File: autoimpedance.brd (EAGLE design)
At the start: 32.1 x 50.8 mm, 42 parts, among them IC1 AD5933, IC2 LM234, IC3 AD5245, Q1 DMG2307L-7

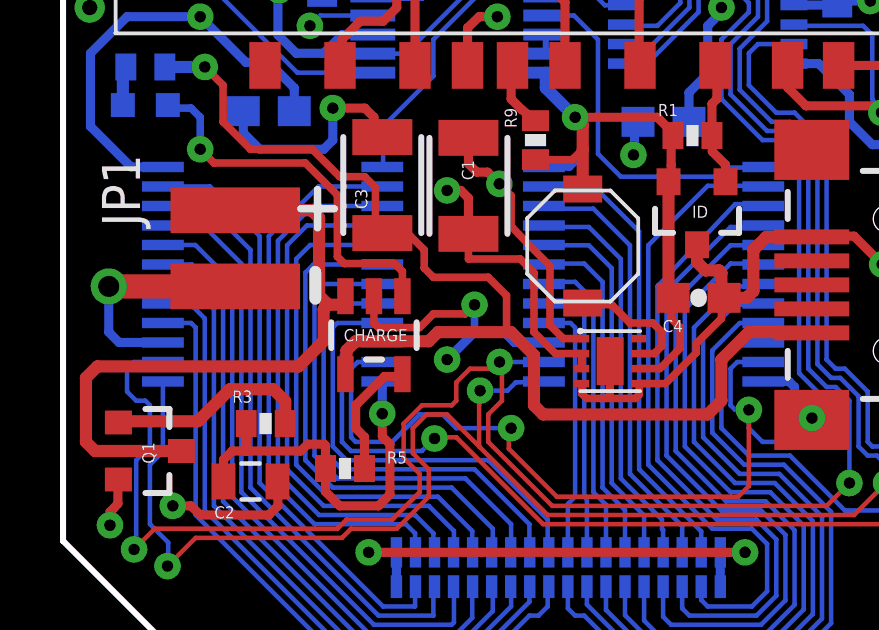
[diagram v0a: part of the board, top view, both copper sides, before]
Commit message: Add Gerber files and .cam
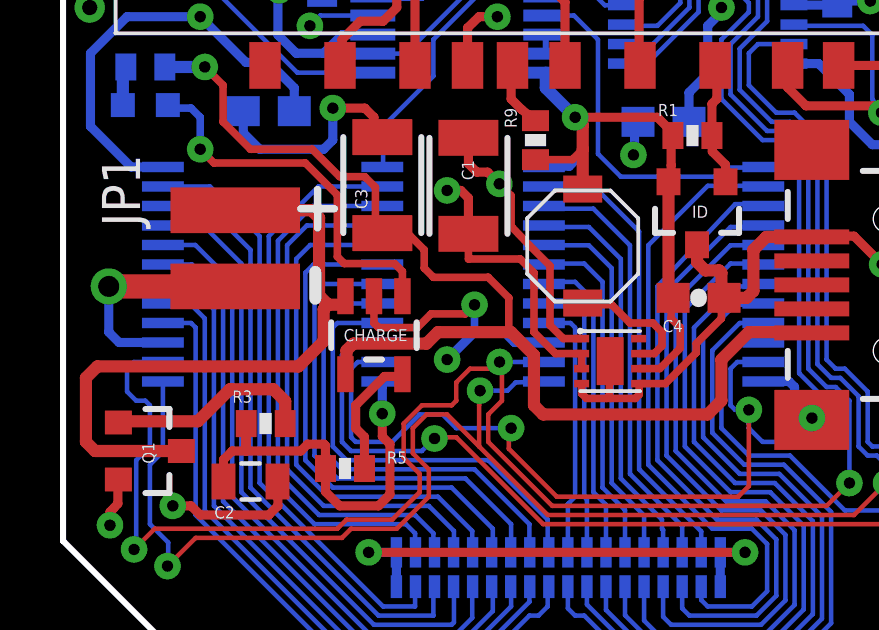
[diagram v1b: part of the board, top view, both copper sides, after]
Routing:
- net VIN: track 27.9 -> 29.5 mm
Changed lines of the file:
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@@
 <layer number="1" name="Top" color="4" fill="1" visible="no" active="yes"/>
 <layer number="2" name="Route2" color="11" fill="1" visible="no" active="yes"/>
-<layer number="3" name="Route3" color="8" fill="1" visible="no" active="yes"/>
+<layer number="3" name="Route3" color="8" fill="1" visible="yes" active="yes"/>
 <layer number="4" name="Route4" color="1" fill="4" visible="no" active="no"/>
 <layer number="5" name="Route5" color="4" fill="4" visible="no" active="no"/>
@@
 <layer number="15" name="Route15" color="4" fill="6" visible="no" active="no"/>
 <layer number="16" name="Bottom" color="1" fill="1" visible="no" active="yes"/>
-<layer number="17" name="Pads" color="2" fill="1" visible="no" active="yes"/>
-<layer number="18" name="Vias" color="2" fill="1" visible="no" active="yes"/>
+<layer number="17" name="Pads" color="2" fill="1" visible="yes" active="yes"/>
+<layer number="18" name="Vias" color="2" fill="1" visible="yes" active="yes"/>
 <layer number="19" name="Unrouted" color="15" fill="1" visible="no" active="yes"/>
 <layer number="20" name="Dimension" color="15" fill="1" visible="no" active="yes"/>
-<layer number="21" name="tPlace" color="3" fill="1" visible="no" active="yes"/>
+<layer number="21" name="tPlace" color="3" fill="1" visible="yes" active="yes"/>
 <layer number="22" name="bPlace" color="5" fill="1" visible="yes" active="yes"/>
 <layer number="23" name="tOrigins" color="15" fill="1" visible="no" active="yes"/>
 <layer number="24" name="bOrigins" color="15" fill="1" visible="no" active="yes"/>
-<layer number="25" name="tNames" color="3" fill="1" visible="no" active="yes"/>
+<layer number="25" name="tNames" color="3" fill="1" visible="yes" active="yes"/>
 <layer number="26" name="bNames" color="5" fill="1" visible="yes" active="yes"/>
-<layer number="27" name="tValues" color="3" fill="1" visible="no" active="yes"/>
+<layer number="27" name="tValues" color="3" fill="1" visible="yes" active="yes"/>
 <layer number="28" name="bValues" color="5" fill="1" visible="yes" active="yes"/>
 <layer number="29" name="tStop" color="7" fill="1" visible="no" active="yes"/>
@@
 <wire x1="10.3632" y1="13.2381" x2="10.3632" y2="12.3444" width="0.254" layer="1"/>
 <wire x1="10.3632" y1="12.3444" x2="10.5156" y2="12.192" width="0.254" layer="1"/>
-<wire x1="10.5156" y1="12.192" x2="11.8872" y2="12.192" width="0.254" layer="1"/>
-<wire x1="11.8872" y1="12.192" x2="12.3444" y2="12.6492" width="0.254" layer="1"/>
-<wire x1="12.3444" y1="12.6492" x2="13.4112" y2="12.6492" width="0.254" layer="1"/>
+<wire x1="10.5156" y1="12.192" x2="11.811" y2="12.192" width="0.254" layer="1"/>
+<wire x1="11.811" y1="12.192" x2="12.2682" y2="12.6492" width="0.254" layer="1"/>
+<wire x1="12.2682" y1="12.6492" x2="13.4112" y2="12.6492" width="0.254" layer="1"/>
 <wire x1="13.4112" y1="12.6492" x2="13.716" y2="12.954" width="0.254" layer="1"/>
 <wire x1="5.7404" y1="13.5636" x2="1.524" y2="13.5636" width="0.8128" layer="1"/>
@@
 <wire x1="15.24" y1="14.478" x2="13.513" y2="14.478" width="0.254" layer="1"/>
 <wire x1="13.513" y1="14.478" x2="13.5128" y2="15.3164" width="0.254" layer="1"/>
-<wire x1="1.5646" y1="5.6032" x2="7.1272" y2="8.956" width="0.6096" layer="3"/>
-<wire x1="7.1272" y1="8.956" x2="12.8016" y2="14.6304" width="0.6096" layer="3"/>
-<wire x1="12.8016" y1="14.6304" x2="12.8016" y2="16.764" width="0.6096" layer="3"/>
+<wire x1="1.5646" y1="5.6032" x2="1.5646" y2="8.3464" width="0.6096" layer="3"/>
+<wire x1="1.5646" y1="8.3464" x2="7.6962" y2="14.478" width="0.6096" layer="3"/>
+<wire x1="7.6962" y1="14.478" x2="11.8872" y2="14.478" width="0.6096" layer="3"/>
+<wire x1="11.8872" y1="14.478" x2="12.8016" y2="15.24" width="0.6096" layer="3"/>
+<wire x1="12.8016" y1="15.24" x2="12.8016" y2="16.764" width="0.6096" layer="3"/>
 <wire x1="13.5128" y1="15.3164" x2="13.5128" y2="16.51" width="0.3048" layer="1"/>
 <wire x1="13.5128" y1="16.51" x2="13.2588" y2="16.764" width="0.3048" layer="1"/>
@@
 <wire x1="3.3932" y1="20.8788" x2="4.7244" y2="20.8788" width="0.4064" layer="16"/>
 <via x="4.7244" y="20.8788" extent="1-16" drill="0.381"/>
-<wire x1="12.192" y1="11.7348" x2="9.7536" y2="11.7348" width="0.4064" layer="1"/>
-<wire x1="9.7536" y1="11.7348" x2="9.4488" y2="11.43" width="0.4064" layer="1"/>
+<wire x1="12.1158" y1="11.6586" x2="9.6774" y2="11.6586" width="0.4064" layer="1"/>
+<wire x1="9.6774" y1="11.6586" x2="9.4488" y2="11.43" width="0.4064" layer="1"/>
 <wire x1="9.4488" y1="11.43" x2="9.4488" y2="10.5211" width="0.4064" layer="1"/>
 <wire x1="9.4488" y1="10.5211" x2="9.4132" y2="10.6379" width="0.4064" layer="1"/>
-<wire x1="12.192" y1="11.7348" x2="12.4968" y2="12.0396" width="0.4064" layer="1"/>
-<wire x1="12.4968" y1="12.0396" x2="14.7828" y2="12.0396" width="0.4064" layer="1"/>
-<wire x1="14.7828" y1="12.0396" x2="14.9352" y2="12.0396" width="0.4064" layer="1"/>
+<wire x1="12.1158" y1="11.6586" x2="12.4968" y2="12.0396" width="0.4064" layer="1"/>
+<wire x1="12.4968" y1="12.0396" x2="14.859" y2="12.0396" width="0.4064" layer="1"/>
+<wire x1="14.859" y1="12.0396" x2="14.9352" y2="12.0396" width="0.4064" layer="1"/>
 <wire x1="14.9352" y1="12.0396" x2="15.6972" y2="11.2776" width="0.4064" layer="1"/>
 <wire x1="15.6972" y1="11.2776" x2="15.6972" y2="9.6012" width="0.4064" layer="1"/>
@@
 <wire x1="12.0396" y1="14.1732" x2="12.3444" y2="13.8684" width="0.254" layer="1"/>
 <wire x1="12.3444" y1="13.8684" x2="14.1732" y2="13.8684" width="0.254" layer="1"/>
-<wire x1="14.1732" y1="13.8684" x2="14.7828" y2="13.2588" width="0.254" layer="1"/>
-<wire x1="14.7828" y1="13.2588" x2="14.7828" y2="12.0396" width="0.254" layer="1"/>
+<wire x1="14.1732" y1="13.8684" x2="14.859" y2="13.1826" width="0.254" layer="1"/>
+<wire x1="14.859" y1="13.1826" x2="14.859" y2="12.0396" width="0.254" layer="1"/>
 <wire x1="10.6426" y1="15.3418" x2="10.414" y2="15.6464" width="0.254" layer="1"/>
 <wire x1="10.414" y1="15.6464" x2="10.414" y2="16.8656" width="0.254" layer="1"/>
